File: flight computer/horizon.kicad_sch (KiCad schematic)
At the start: 38 parts, among them J2 Conn_02x03_Counter_Clockwise, J7 Conn_02x03_Counter_Clockwise, J8 Conn_02x03_Counter_Clockwise, SW1 CK_KMS2xxG, U1 MMCU, U2 MKL02Z32VFG4, U3 NMCU, U4 TMCU, Y1 Crystal

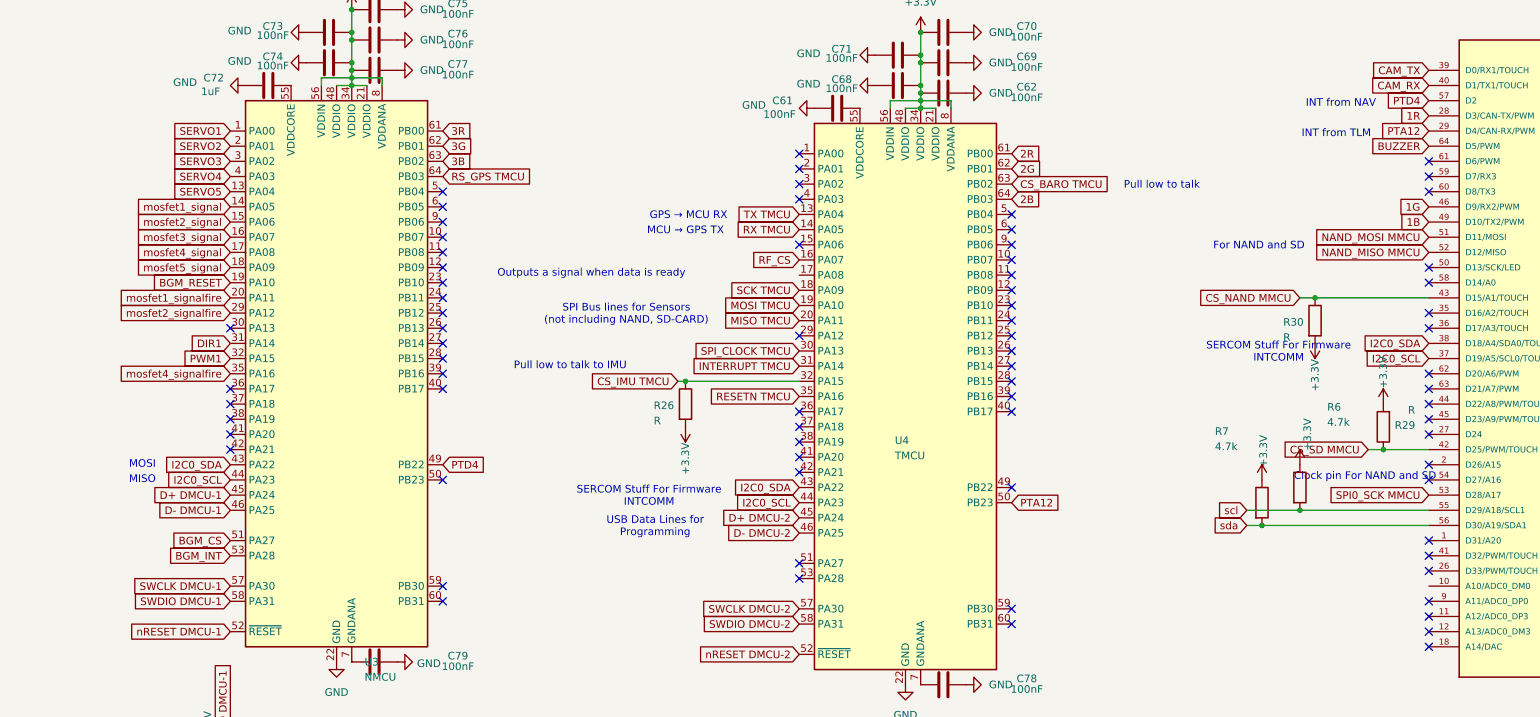
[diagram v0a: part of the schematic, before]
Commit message: a few small changes to make cyao happy!
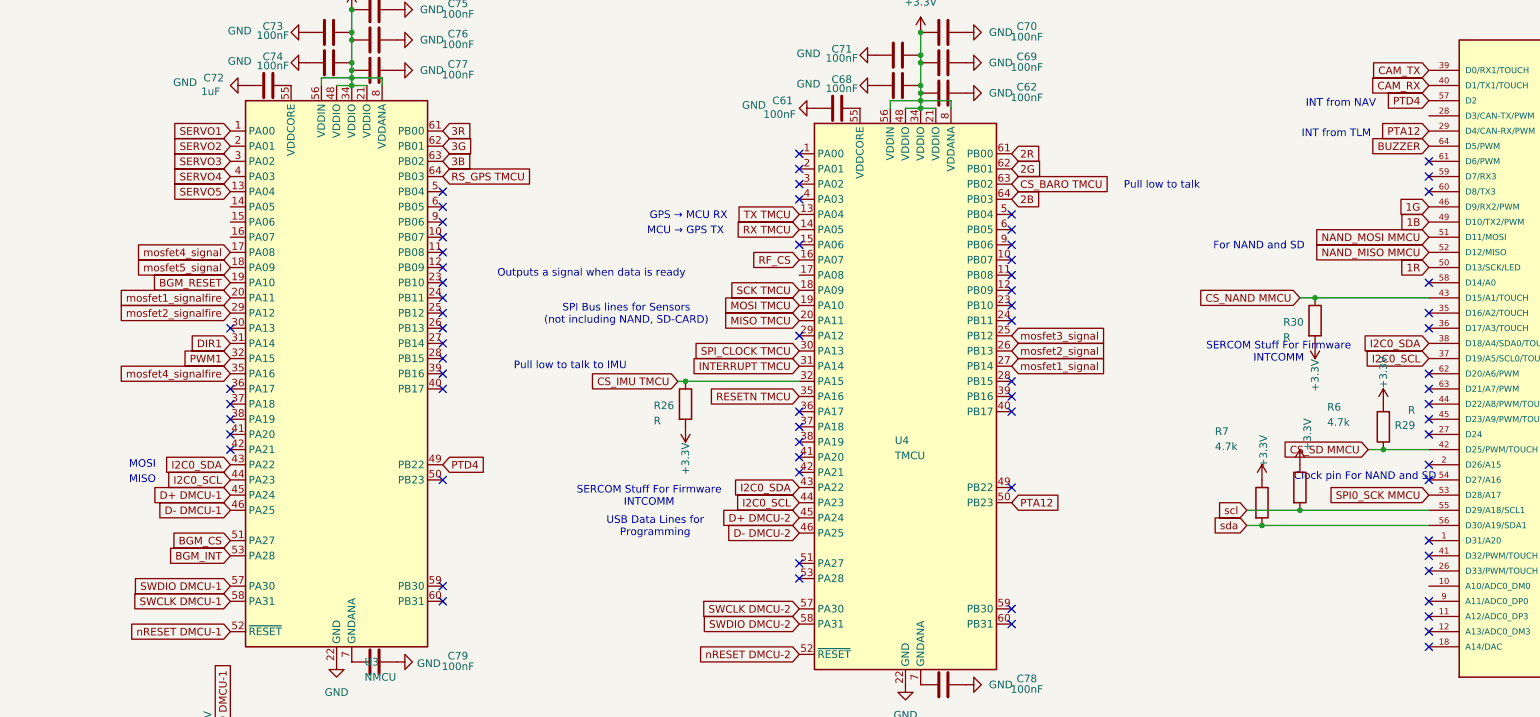
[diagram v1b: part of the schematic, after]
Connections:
- net 1R: now also U1.50 (D13/SCK/LED); no longer U1.28 (D3/CAN-TX/PWM)
- net SWCLK DMCU-1: now also U3.58 (PA31); no longer U3.57 (PA30)
- net SWDIO DMCU-1: now also U3.57 (PA30); no longer U3.58 (PA31)
- net mosfet1_signal: now also U4.27 (PB14); no longer U3.14 (PA05)
- net mosfet2_signal: now also U4.26 (PB13); no longer U3.15 (PA06)
- net mosfet3_signal: now also U4.25 (PB12); no longer U3.16 (PA07)
- no-connect marks 77 -> 73
